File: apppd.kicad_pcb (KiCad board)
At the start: 2 copper layers, 59 parts, among them J1 Conn_SWD, J2 APPPD Connector, J4 2601-1102, J5 USB_C_Receptacle_USB2.0_16P, Q1 AO3400A, Q2 AO3400A, SW1 NRST, SW2 BOOT0, U1 AP2112K-3.3, U2 STM32F072CBTx, U3 USBLC6-2SC6, U4 TCAN337, U5 SN74LVC2G14DBVR

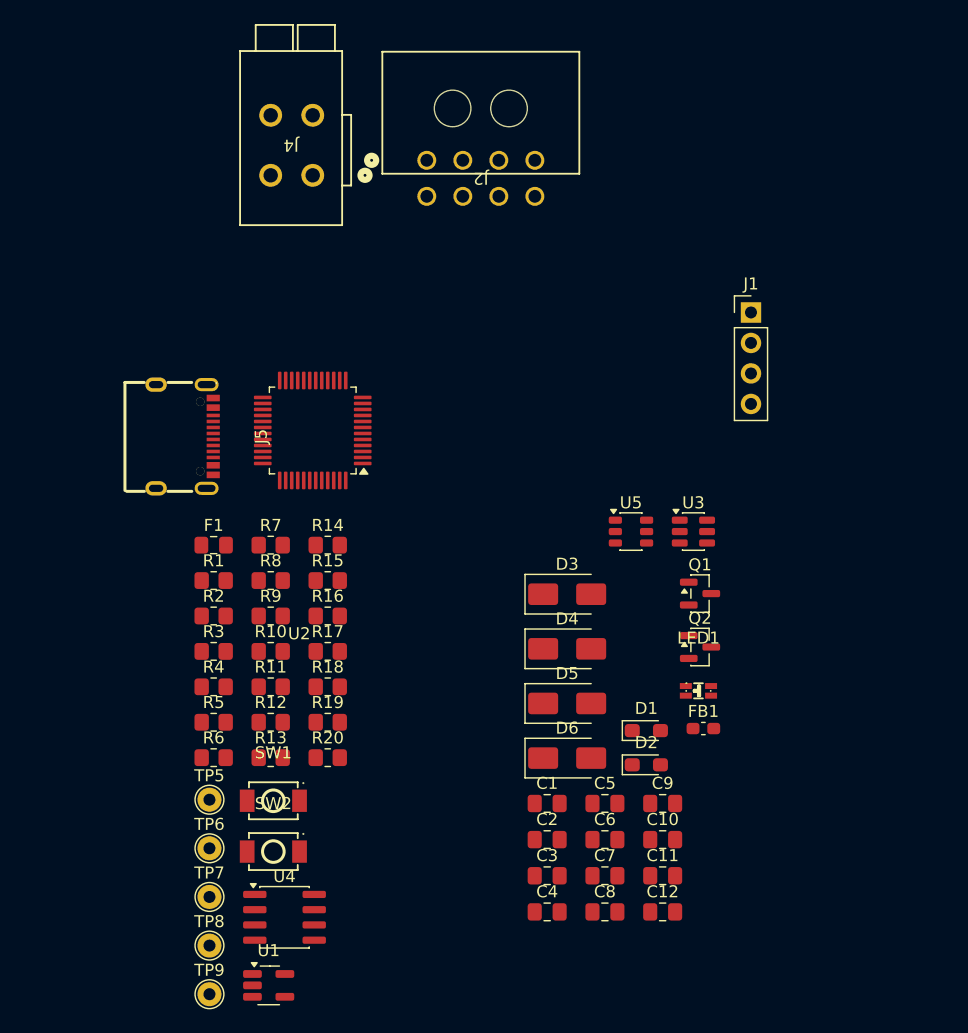
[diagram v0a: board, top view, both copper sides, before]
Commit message: update
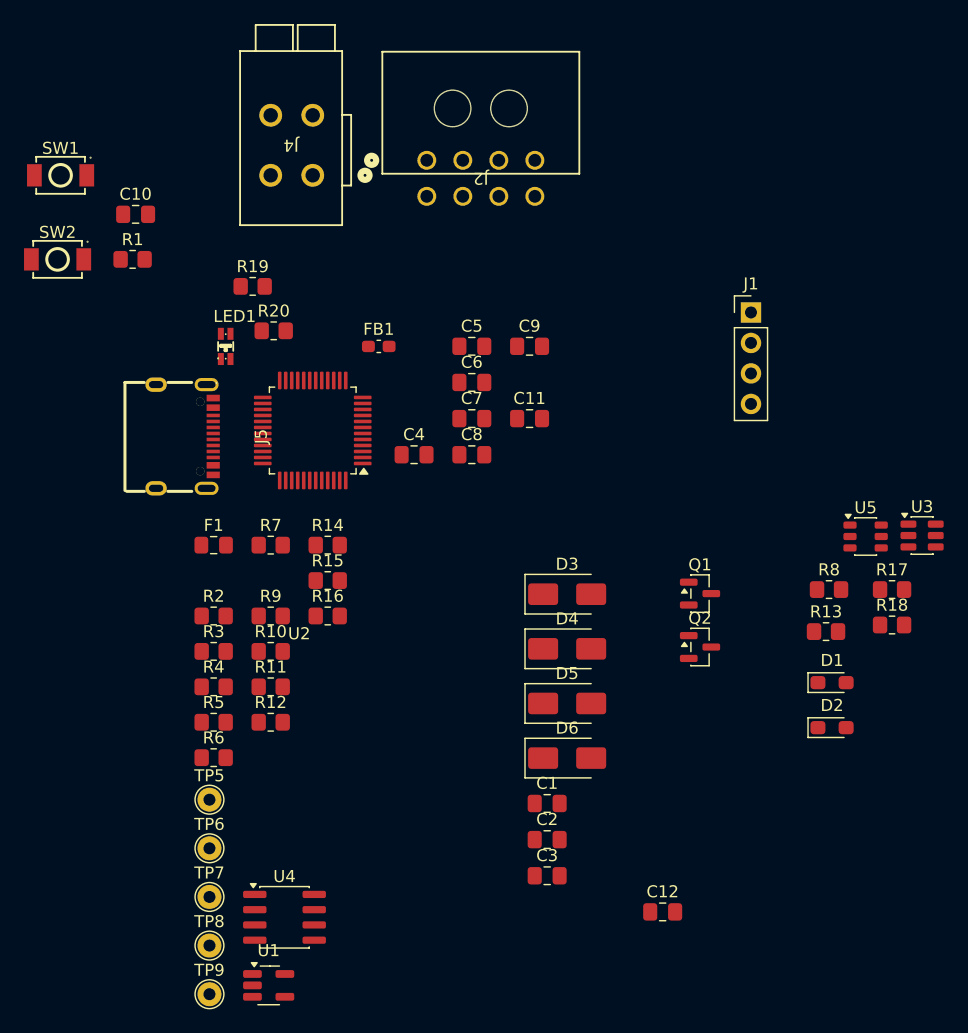
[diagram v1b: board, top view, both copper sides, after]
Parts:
- moved C10 68.1 mm to (25.8, 25.5)
- moved SW1 55.0 mm to (19.5, 22.2)
- moved SW2 52.5 mm to (19.2, 29.2)
- moved LED1 48.7 mm to (33.2, 36.5), turned to 90 degrees
- moved R13 47.4 mm to (83.2, 60.2)
- moved R17 47.3 mm to (88.8, 56.8)
- moved R18 47.3 mm to (88.8, 59.7)
- moved R8 46.5 mm to (83.5, 56.8)
- moved FB1 41.8 mm to (46.0, 36.5)
- moved C6 39.7 mm to (53.8, 39.5)
- moved C11 39.7 mm to (58.6, 42.5)
- moved C4 39.7 mm to (48.9, 45.5)
- moved C5 39.7 mm to (53.8, 36.5)
- moved C7 39.7 mm to (53.8, 42.5)
- moved C8 39.7 mm to (53.8, 45.5)
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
